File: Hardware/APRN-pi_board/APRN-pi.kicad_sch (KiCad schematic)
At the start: 35 parts, among them J1 Raspberry_Pi_2_3, J2 Conn_Coaxial, J3 Amplifier Jumper, J4 Screw_Terminal_01x02, J5 AudioJack4, J6 Conn_01x04, Q1 MMBT3906, Q2 MMBT3906, U1 DRA818V, U2 L7805

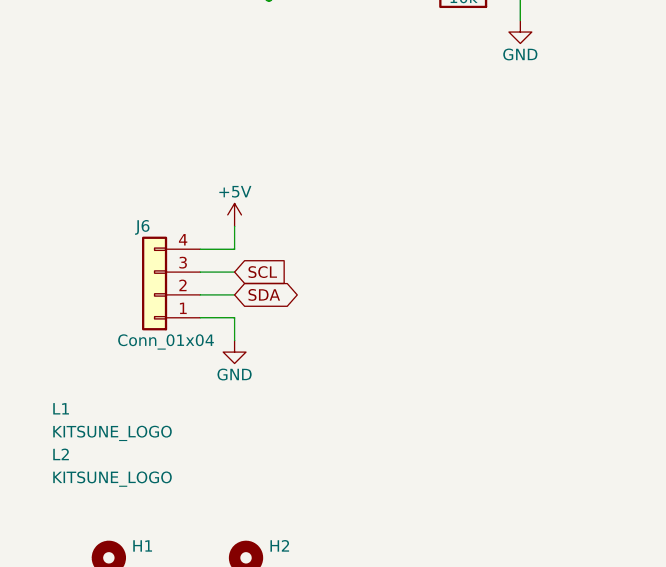
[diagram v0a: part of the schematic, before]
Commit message: Use upstream
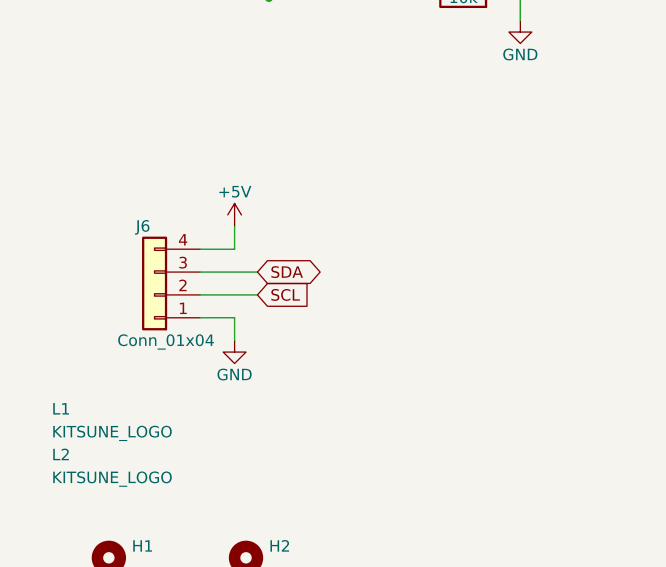
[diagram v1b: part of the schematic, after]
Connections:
- net SCL: now also J6.2 (Pin_2); no longer J6.3 (Pin_3)
- net SDA: now also J6.3 (Pin_3); no longer J6.2 (Pin_2)
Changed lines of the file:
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@@
-    (stroke (width 0) (type default) (color 0 0 0 0))
-  )
-  (wire (pts (xy 31.75 154.94) (xy 35.56 154.94))
     (stroke (width 0) (type default) (color 0 0 0 0))
   )
@@
     (stroke (width 0) (type default) (color 0 0 0 0))
   )
-  (wire (pts (xy 31.75 152.4) (xy 35.56 152.4))
-    (stroke (width 0) (type default) (color 0 0 0 0))
-  )
   (wire (pts (xy 242.57 31.75) (xy 257.81 31.75))
     (stroke (width 0) (type default) (color 0 0 0 0))
@@
     (stroke (width 0) (type default) (color 0 0 0 0))
   )
+  (wire (pts (xy 31.75 152.4) (xy 38.1 152.4))
+    (stroke (width 0) (type default) (color 0 0 0 0))
+  )
   (wire (pts (xy 31.75 149.86) (xy 35.56 149.86))
     (stroke (width 0) (type default) (color 0 0 0 0))
@@
   )
   (wire (pts (xy 139.7 139.7) (xy 147.32 139.7))
+    (stroke (width 0) (type default) (color 0 0 0 0))
+  )
+  (wire (pts (xy 31.75 154.94) (xy 38.1 154.94))
     (stroke (width 0) (type default) (color 0 0 0 0))
   )
@@
     )
   )
-  (global_label "SDA" (shape bidirectional) (at 35.56 154.94 0) (fields_autoplaced)
+  (global_label "SDA" (shape bidirectional) (at 38.1 152.4 0) (fields_autoplaced)
     (effects (font (size 1.27 1.27)) (justify left))
-    (property "Intersheet References" "${INTERSHEET_REFS}" (id 0) (at 41.5412 154.8606 0)
+    (property "Intersheet References" "${INTERSHEET_REFS}" (id 0) (at 44.0812 152.3206 0)
       (effects (font (size 1.27 1.27)) (justify left) hide)
     )
@@
     )
   )
-  (global_label "SCL" (shape input) (at 35.56 152.4 0) (fields_autoplaced)
+  (global_label "SCL" (shape input) (at 38.1 154.94 0) (fields_autoplaced)
     (effects (font (size 1.27 1.27)) (justify left))
-    (property "Intersheet References" "${INTERSHEET_REFS}" (id 0) (at 41.4807 152.3206 0)
+    (property "Intersheet References" "${INTERSHEET_REFS}" (id 0) (at 44.0207 154.8606 0)
       (effects (font (size 1.27 1.27)) (justify left) hide)
     )
